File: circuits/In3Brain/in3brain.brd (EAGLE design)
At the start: 42.2 x 38.2 mm, 21 parts, among them IC1 ATMEGA48/88/168-AU, IC2 REG1117

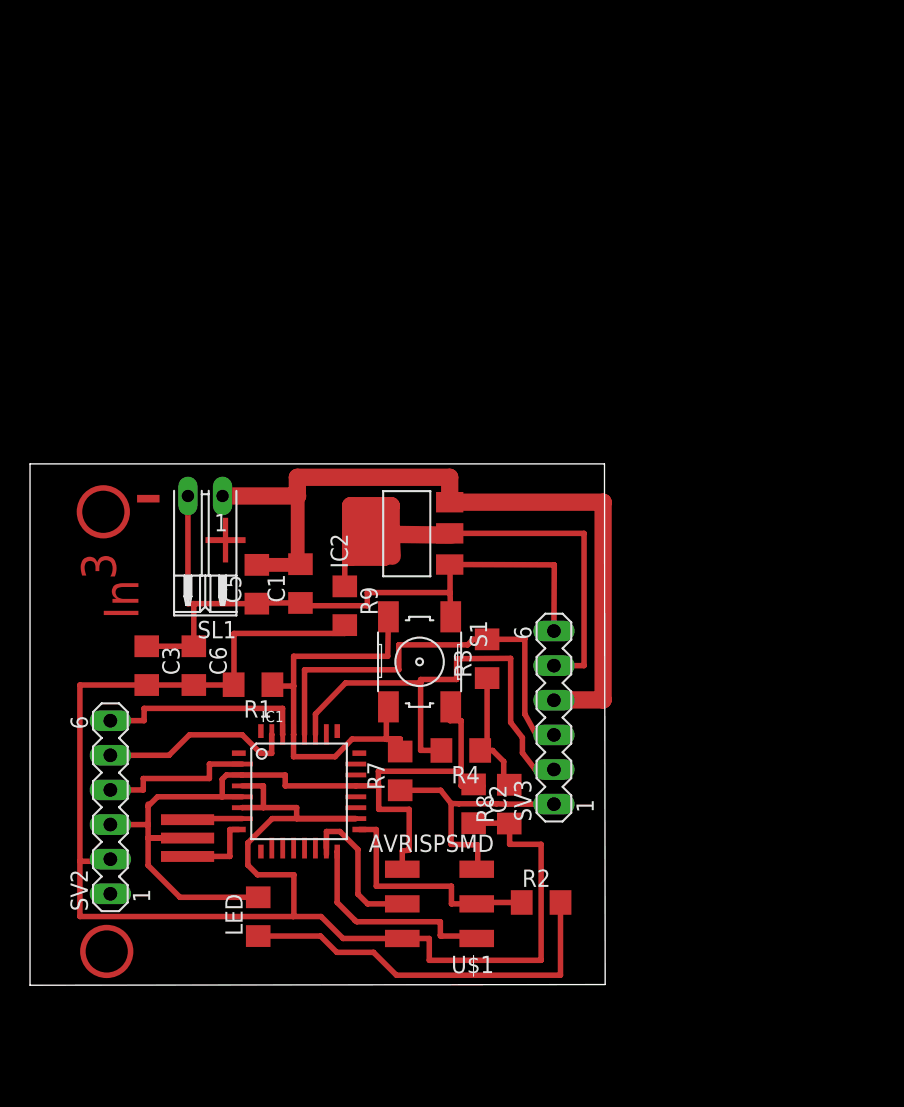
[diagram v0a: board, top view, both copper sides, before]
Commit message: Electronics v2
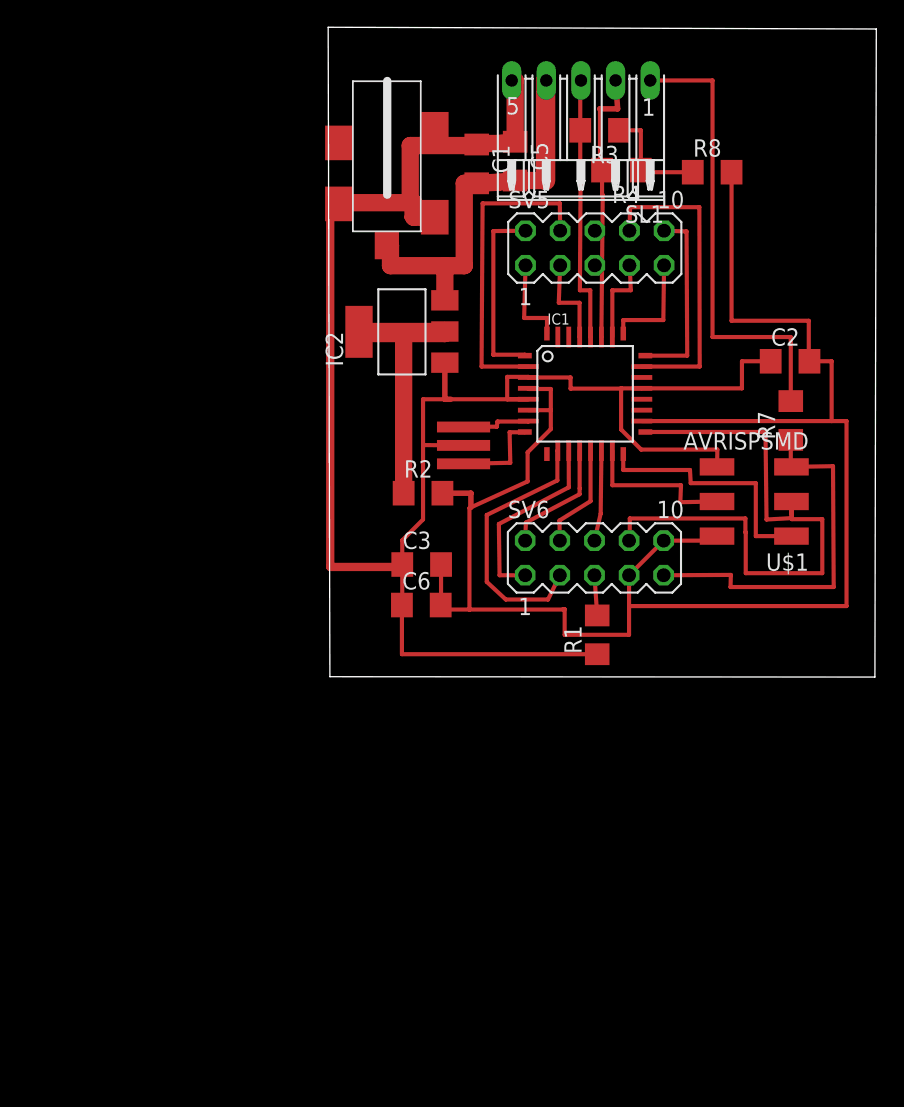
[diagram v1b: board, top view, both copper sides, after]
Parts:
- removed LED: (no value), ng:1206
- removed R9: 0, ng:1206
- removed S1: (no value), ng:6MM_SWITCH
- removed SV2, SV3: (no value), con-lstb:MA06-1
- added J1: JACK.65MM, 01_fab:JACK_.65MM
- added SV5, SV6: (no value), con-lstb:MA05-2
- R1: value 10k -> 0
- R2: value 499 -> 0
- SL1: device con-amp-quick:02PA -> con-amp-quick:05PA
- moved R8 48.7 mm to (49.9, 59.4), turned to 0 degrees
- moved R4 44.2 mm to (43.3, 59.6)
- moved SL1 41.1 mm to (40.3, 66.1)
- moved C2 39.9 mm to (55.6, 45.5), turned to 0 degrees
- moved R3 39.6 mm to (41.7, 62.5), turned to 180 degrees
- moved R7 38.5 mm to (55.7, 41.2)
- moved U$1 37.5 mm to (53.2, 35.3)
- moved C5 36.4 mm to (35.5, 60.2), turned to 270 degrees
- moved IC1 35.9 mm to (40.6, 43.2)
- moved U$2 35.2 mm to (31.7, 39.4)
- moved C1 33.4 mm to (32.6, 60.0), turned to 270 degrees
- moved R2 31.2 mm to (28.7, 35.9)
- moved R1 25.5 mm to (41.5, 25.5), turned to 90 degrees
- moved C3 21.5 mm to (28.6, 30.6), turned to 0 degrees
- moved C6 17.3 mm to (28.6, 27.7), turned to 0 degrees
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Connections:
- removed net EN: SV2.1
- removed net N$23: LED.1, R2.2
- new net $1: SV5.5
- new net $2: SV5.6
- new net BTN: IC1.2, SV5.4
- new net BUZZ: IC1.12, SV6.2
- new net INT0: IC1.32, SV5.1
- new net INT1: IC1.1, SV5.2
- new net LCD4: IC1.23, SV5.8
- new net LCD5: IC1.24, SV5.10
- new net LCD6: IC1.25, SV5.9
- new net LCD7: IC1.26, SV5.7
- new net LCDE: IC1.10, SV6.3
- new net LCDRS: IC1.11, SV6.1
- new net RGBB: IC1.14, SV6.6
- new net RGBG: IC1.13, SV6.4
- net 12V: now also J1.PIN, SL1.4; no longer SL1.1, SV3.4
- net 5V: now also R2.1, R2.2, SV6.10, SV6.7; no longer R1.2, R9.1, R9.2, SV2.2, SV3.5
- net GND: now also J1.CONTACT, J1.SHUNT, R1.1, R1.2, SL1.5, SV6.5; no longer LED.2, S1.1, S1.2, SL1.2, SV2.3, SV3.6
- net RST: now also SL1.1, SV5.3, SV6.9; no longer R1.1, S1.3, S1.4, SV3.1
- net RX: no longer SV2.6
- net SCK: now also SV6.8; no longer R2.1
- net SCL: now also SL1.3; no longer SV3.3
- net SDA: now also SL1.2; no longer SV3.2
- net STATE: now also IC1.9; no longer IC1.2, SV2.4
- net TX: no longer SV2.5
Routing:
- net GND: track 119.2 -> 154.0 mm
- net 12V: track 58.7 -> 29.1 mm
- net N$23: track 28.7 -> 0.00 mm
- net SCK: track 18.0 -> 46.6 mm
- net BTN: track 0.00 -> 23.1 mm
- net LCD4: track 0.00 -> 22.8 mm
- net LCDE: track 0.00 -> 19.9 mm
- net N$3: track 18.5 -> 0.00 mm
- net RST: track 50.3 -> 68.1 mm
- net RX: track 15.5 -> 0.00 mm
- net SDA: track 35.2 -> 20.3 mm
- net TX: track 14.4 -> 0.00 mm
- net LCDRS: track 0.00 -> 14.1 mm
- net LCD5: track 0.00 -> 13.8 mm
- net INT1: track 0.00 -> 13.8 mm
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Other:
- board size 42.2 x 38.2 mm -> 40.2 x 47.7 mm
- board text removed: "+"
- board text removed: "-"
- board text removed: "3"
- board text removed: "In"

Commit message: New Electronics
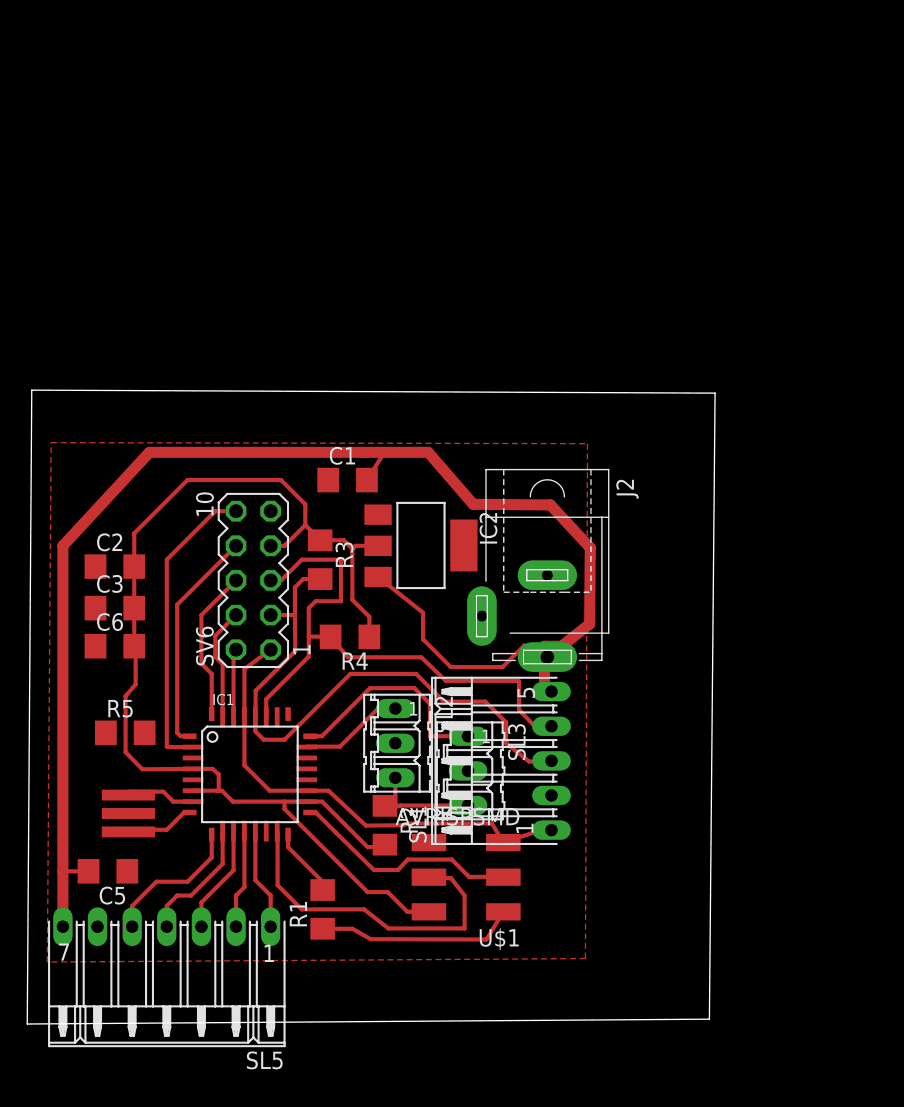
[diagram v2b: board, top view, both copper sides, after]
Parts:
- removed J1: JACK.65MM, 01_fab:JACK_.65MM
- removed R7, R8: 0, ng:1206
- removed SV5: (no value), con-lstb:MA05-2
- added J2: (no value), con-jack:SPC4078
- added R5: 0, ng:1206
- added SL2, SL3: (no value), con-amp-quick:03P
- added SL5: (no value), con-amp-quick:07PA
- moved C5 60.1 mm to (5.59, 8.13), turned to 180 degrees
- moved C2 51.8 mm to (6.10, 30.5)
- moved SL1 50.0 mm to (38.1, 16.2), turned to 90 degrees
- moved R4 39.6 mm to (23.3, 25.3)
- moved R3 37.6 mm to (21.2, 31.0), turned to 270 degrees
- moved IC1 37.2 mm to (16.0, 15.2)
- moved U$2 36.5 mm to (7.09, 12.4)
- moved U$1 34.7 mm to (32.1, 7.70)
- moved R1 28.5 mm to (21.3, 5.33)
- moved SV6 25.1 mm to (16.3, 29.5), turned to 90 degrees
- moved C1 25.1 mm to (23.2, 36.8), turned to 0 degrees
- moved R2 24.5 mm to (25.9, 11.5), turned to 270 degrees
- moved C3 22.7 mm to (6.10, 27.4)
- moved C6 22.7 mm to (6.10, 24.6)
- moved IC2 15.7 mm to (28.5, 32.0), turned to 270 degrees
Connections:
- removed net $1: SV5.5
- removed net $2: SV5.6
- removed net LCD4: IC1.23, SV5.8
- removed net LCD5: IC1.24, SV5.10
- removed net LCD6: IC1.25, SV5.9
- removed net LCD7: IC1.26, SV5.7
- removed net LCDE: IC1.10, SV6.3
- removed net LCDRS: IC1.11, SV6.1
- removed net RGBB: IC1.14, SV6.6
- removed net RGBG: IC1.13, SV6.4
- removed net RX: IC1.30
- removed net STATE: IC1.9
- removed net TX: IC1.31
- new net FAN12: IC1.9, SL5.5
- new net FAN5: IC1.10, SL5.4
- new net LED: IC1.2, SV6.10
- new net PUMP: IC1.13, SL5.1
- new net RELAY1: IC1.11, SL5.3
- new net RELAY2: IC1.12, SL5.2
- new net TEMP1: IC1.23, SL2.1
- new net TEMP2: IC1.24, SL3.1
- net 12V: now also J2.3, SL1.5, SL5.7; no longer J1.PIN, SL1.4
- net 5V: now also SL2.3, SL3.3; no longer R8.1, R8.2, SV6.10
- net BTN: now also IC1.31, SV6.4; no longer IC1.2, SV5.4
- net BUZZ: now also IC1.30; no longer IC1.12
- net GND: now also J2.1, J2.2, R5.1, R5.2, SL1.2, SL2.2, SL3.2, SL5.6, SV6.9; no longer J1.CONTACT, J1.SHUNT, R1.1, R1.2, SL1.5, SV6.5
- net INT0: now also IC1.1, SV6.8; no longer IC1.32, SV5.1
- net INT1: now also IC1.32, SV6.6; no longer IC1.1, SV5.2
- net MISO: now also R1.1, R1.2
- net RST: now also IC1.19, SV6.1; no longer R7.1, R7.2, SV5.3, SV6.9
- net SCK: no longer SV6.8
- net SCL: now also SV6.3
- net SDA: now also SL1.4, SV6.5; no longer SL1.2
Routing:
- net GND: track 154.0 -> 0.00 mm
- net 12V: track 29.1 -> 111.4 mm
- net 5V: track 157.2 -> 98.2 mm
- net RST: track 68.1 -> 34.7 mm
- net SCK: track 46.6 -> 16.8 mm
- net SCL: track 19.7 -> 43.1 mm
- net LCD4: track 22.8 -> 0.00 mm
- net LED: track 0.00 -> 22.2 mm
- net SDA: track 20.3 -> 42.5 mm
- net LCDE: track 19.9 -> 0.00 mm
- net TEMP2: track 0.00 -> 15.9 mm
- net BTN: track 23.1 -> 8.37 mm
- net LCDRS: track 14.1 -> 0.00 mm
- net LCD5: track 13.8 -> 0.00 mm
- net MOSI: track 11.5 -> 24.5 mm
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- added copper zone on layer 1, net GND
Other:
- board size 40.2 x 47.7 mm -> 50.5 x 46.5 mm
